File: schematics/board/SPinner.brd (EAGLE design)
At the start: 63.6 x 63.6 mm, 8 parts

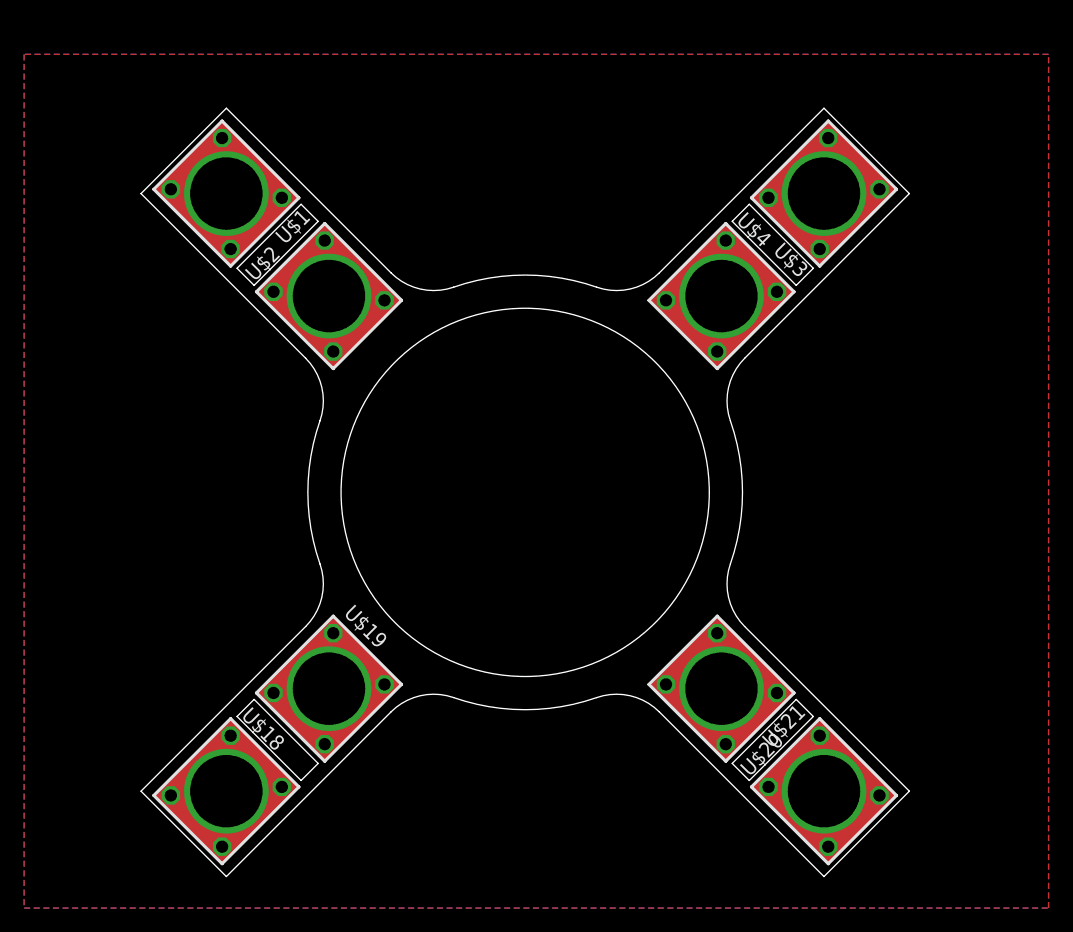
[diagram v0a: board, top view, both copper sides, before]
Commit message: Платы СБ
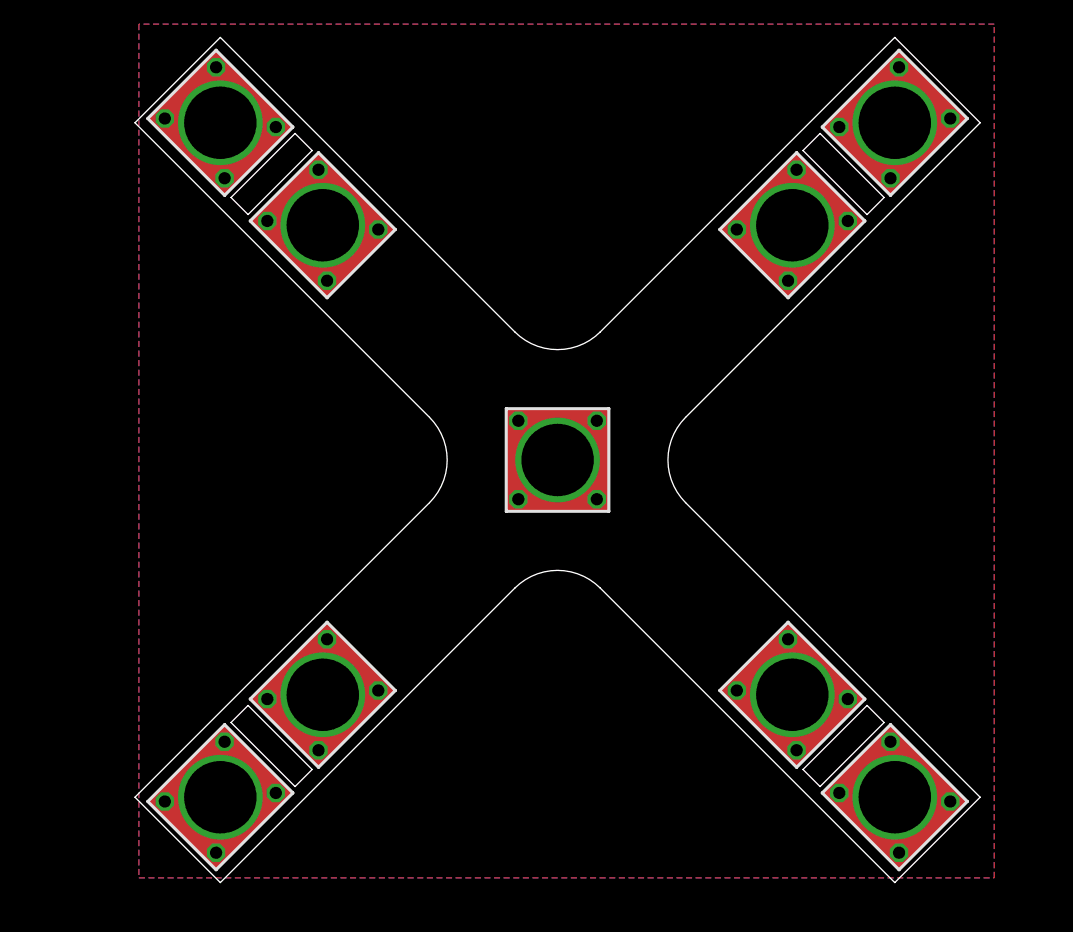
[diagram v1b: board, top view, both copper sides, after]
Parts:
- added U$5: KCONNECTQUAD, CanCubeSat:KCONNECT_QUAD
- moved U$4 8.30 mm to (54.4, 54.4)
- moved U$3 8.29 mm to (62.9, 62.9)
- moved U$2 5.89 mm to (15.6, 54.4)
- moved U$21 5.89 mm to (54.4, 15.6)
- moved U$1 5.88 mm to (7.07, 62.9)
- moved U$20 5.88 mm to (62.9, 7.07)
- moved U$19 0.72 mm to (15.6, 15.6)
- moved U$18 0.71 mm to (7.07, 7.07)
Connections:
- new net CMD: U$5.1, U$5.2, U$5.3, U$5.4, U$5.P$1, U$5.P$2
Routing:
- net BUS+1: track 75.4 -> 0.00 mm
- net CMD: track 0.00 -> 18.4 mm
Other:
- board size 63.6 x 63.6 mm -> 70 x 70 mm
